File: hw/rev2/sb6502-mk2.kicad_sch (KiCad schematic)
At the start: 0 parts

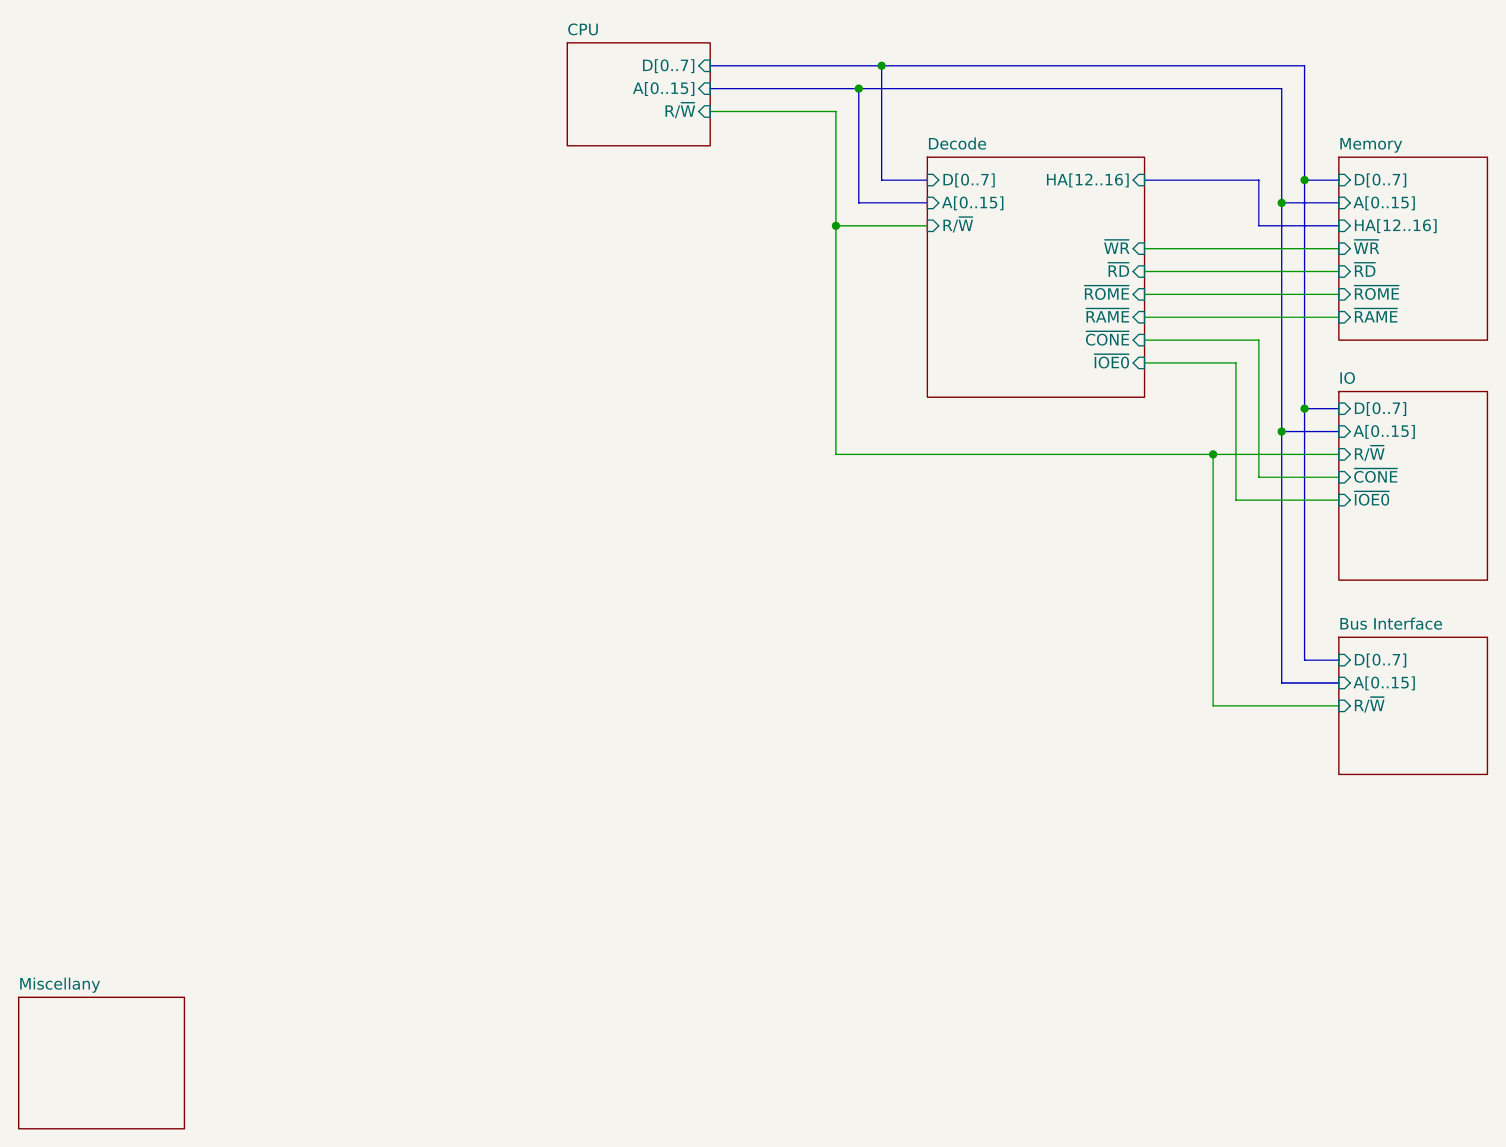
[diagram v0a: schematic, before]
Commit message: more work towards PCB-based design
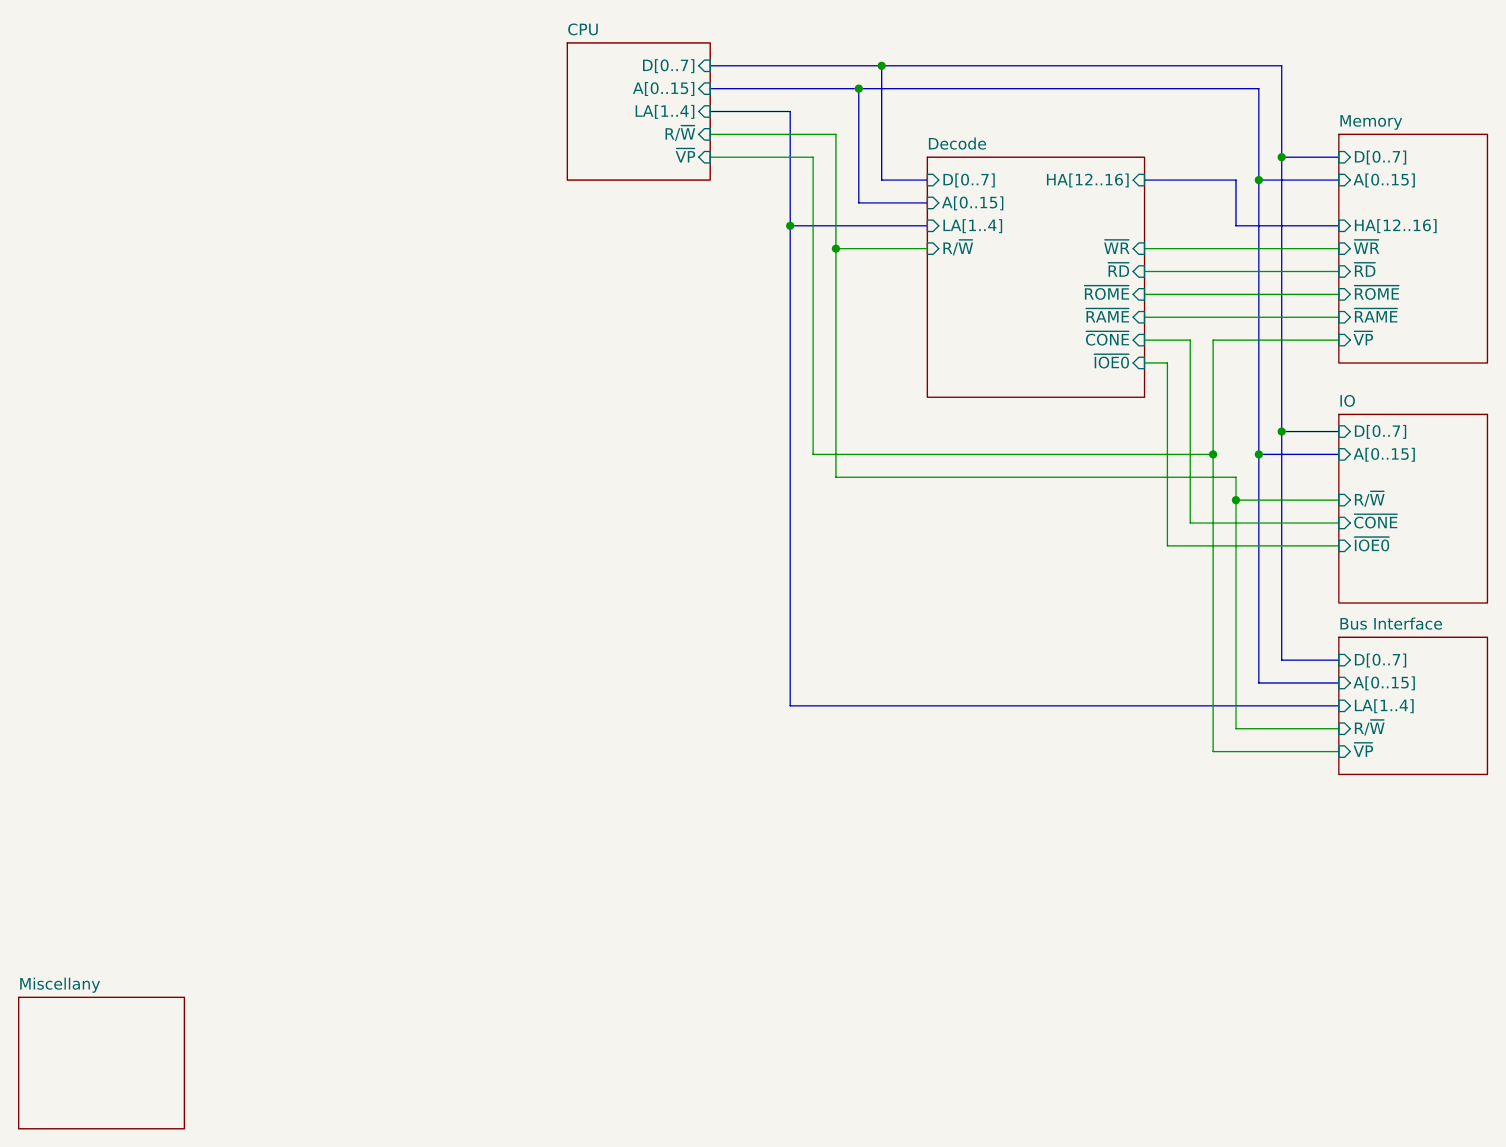
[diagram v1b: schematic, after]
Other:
- sheet Bus Interface ports: added LA[1..4], ~{VP}; removed none
- sheet CPU ports: added LA[1..4], ~{VP}; removed none
- sheet Decode ports: added LA[1..4]; removed none
- sheet Memory ports: added ~{VP}; removed none
